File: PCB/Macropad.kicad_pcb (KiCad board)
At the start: 2 copper layers, 89.5 x 70 mm, 30 parts, among them J1 OLED_128x32, SW1 RotaryEncoder_Switch, SW2 RotaryEncoder_Switch, U1 MOUDLE-SEEEDUINO-XIAO

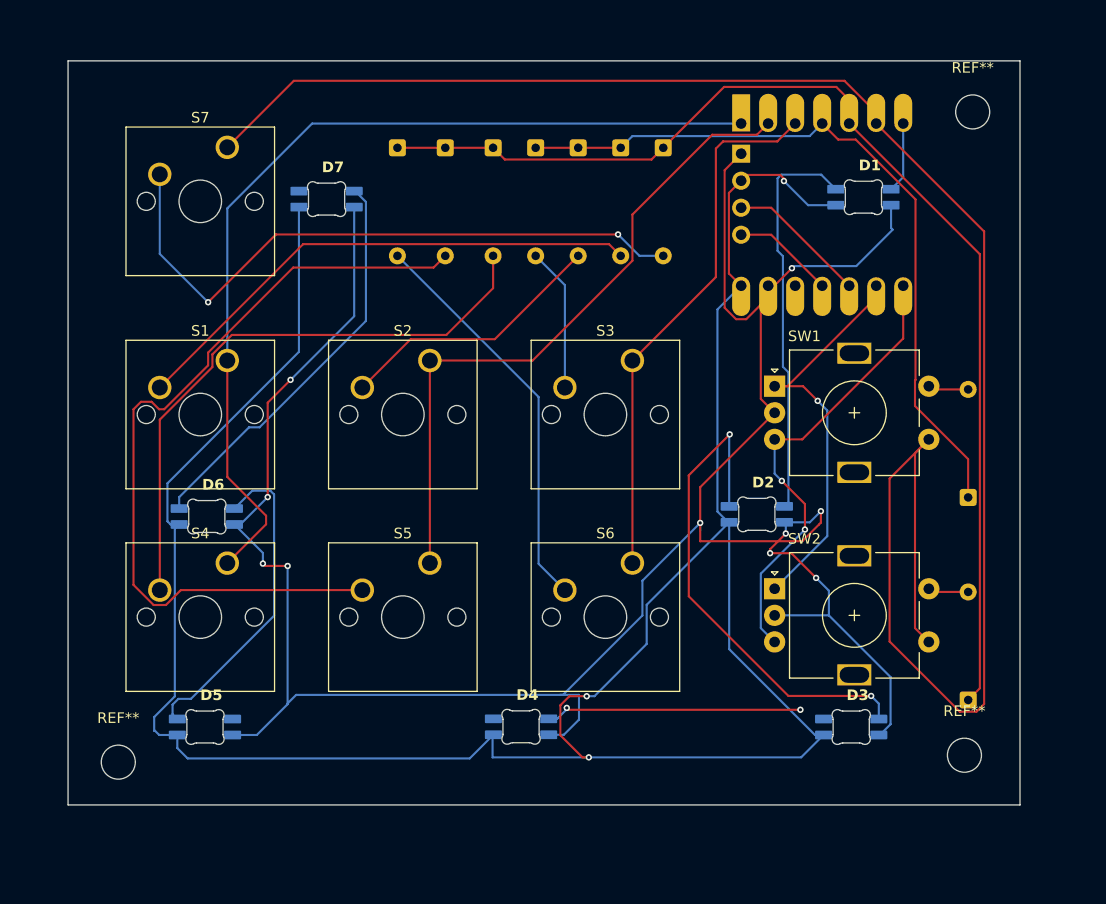
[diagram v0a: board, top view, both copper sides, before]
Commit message: replalced exxisting files
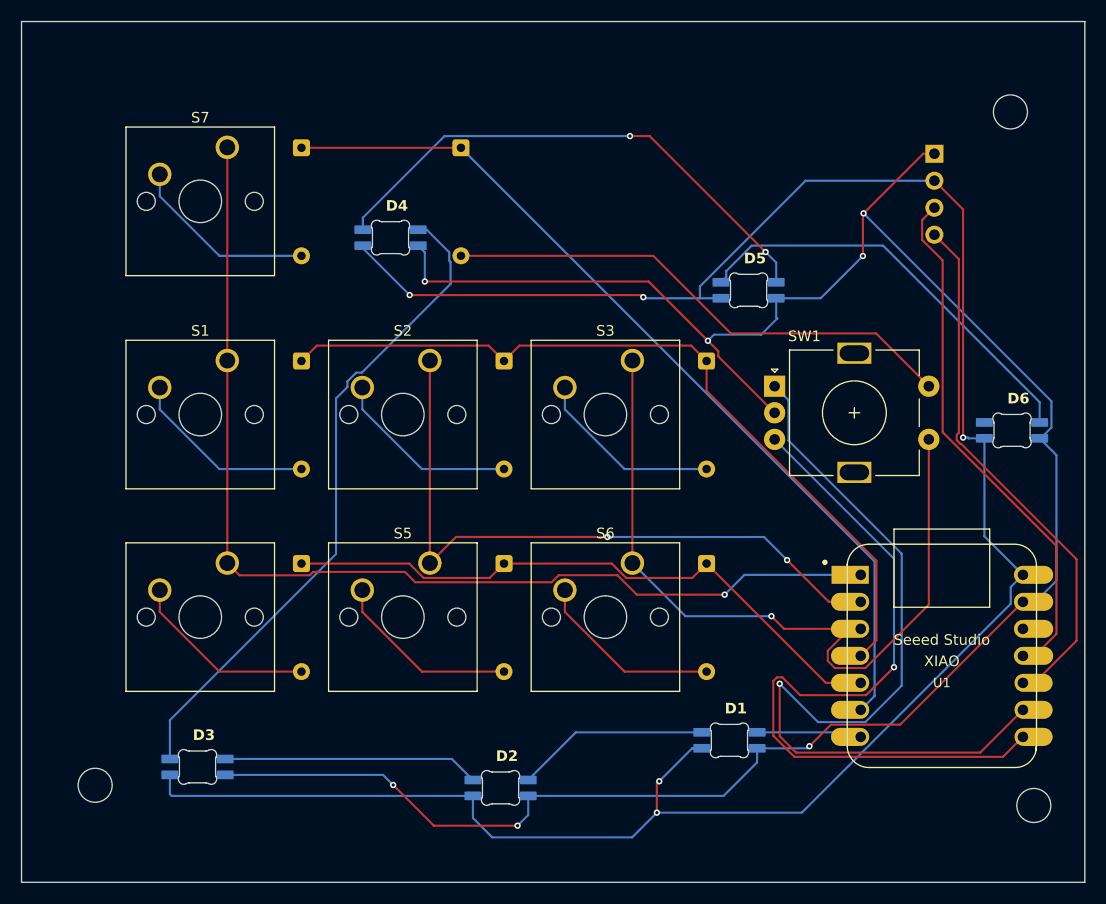
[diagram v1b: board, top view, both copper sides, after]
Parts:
- removed D7: SK6812MINI-E, footprints:SK6812MINI-E_fixed
- removed DI22: ~, Diode_THT:D_DO-35_SOD27_P10.16mm_Horizontal
- removed SW2: RotaryEncoder_Switch, Rotary_Encoder:RotaryEncoder_Alps_EC11E-Switch_Vertical_H20mm
- U1: moved to F.Cu
- moved D6 76.2 mm to (186.4, 67.2)
- moved D5 65.6 mm to (161.7, 54.0)
- moved D3 61.6 mm to (109.8, 98.9)
- moved DI11 57.9 mm to (134.6, 40.5), turned to -90 degrees
- moved D1 52.6 mm to (159.9, 96.4)
- moved DI6 48.7 mm to (157.7, 79.6)
- moved D4 47.6 mm to (128.0, 49.1)
- moved U1 43.9 mm to (179.8, 88.3), turned to 0 degrees
- moved DI4 43.1 mm to (119.6, 79.6)
- moved DI5 39.5 mm to (138.7, 79.6)
- moved DI1 36.1 mm to (119.6, 60.6)
- moved D2 35.3 mm to (138.3, 100.8)
- moved DI7 34.0 mm to (119.6, 40.5)
- moved DI3 25.7 mm to (157.7, 60.6)
- moved DI2 21.2 mm to (138.7, 60.6)
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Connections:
- D6 pad 1: Net-(D6-DOUT) -> unconnected-(D6-DOUT-Pad1)
- DI11 pad 1: Row 0 -> Row
- DI7 pad 1: Row 1 -> Row
- S7 pad 1: Column 3 -> Column 0
- SW1 pad S1: Column 3 -> Column 2
- U1 pad 10: SCL -> SDA
- U1 pad 11: SDA -> SCL
- U1 pad 6: Column 3 -> Row
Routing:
- net Column 3: track 177.3 -> 0.00 mm
- net Row: track 0.00 -> 84.5 mm
- net Net-(DI5-A): track 76.0 -> 17.7 mm
- net Net-(D4-DOUT): track 0.00 -> 50.0 mm, vias 0 -> 2
- net Row 1: track 108.3 -> 59.5 mm
- net Net-(DI11-A): track 3.82 -> 49.1 mm
- net Net-(DI7-A): track 60.2 -> 17.7 mm, vias 2 -> 0
- net SDA: track 9.61 -> 50.6 mm
- net GPIO9: track 38.8 -> 77.6 mm
- net Net-(DI4-A): track 56.2 -> 17.7 mm
- net Net-(D3-DOUT): track 24.3 -> 62.8 mm, vias 2 -> 0
- net Net-(D6-DOUT): track 38.2 -> 0.00 mm
- net SCL: track 13.2 -> 49.8 mm
- net Net-(DI1-A): track 49.4 -> 17.7 mm
- net GPIO8: track 43.5 -> 69.6 mm, vias 2 -> 1
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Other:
- board size 89.5 x 70 mm -> 100 x 80.9 mm
